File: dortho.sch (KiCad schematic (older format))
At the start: 15 parts, among them SW1 SW_Push, U1 ATmega32U4-AU, Y1 16MHz

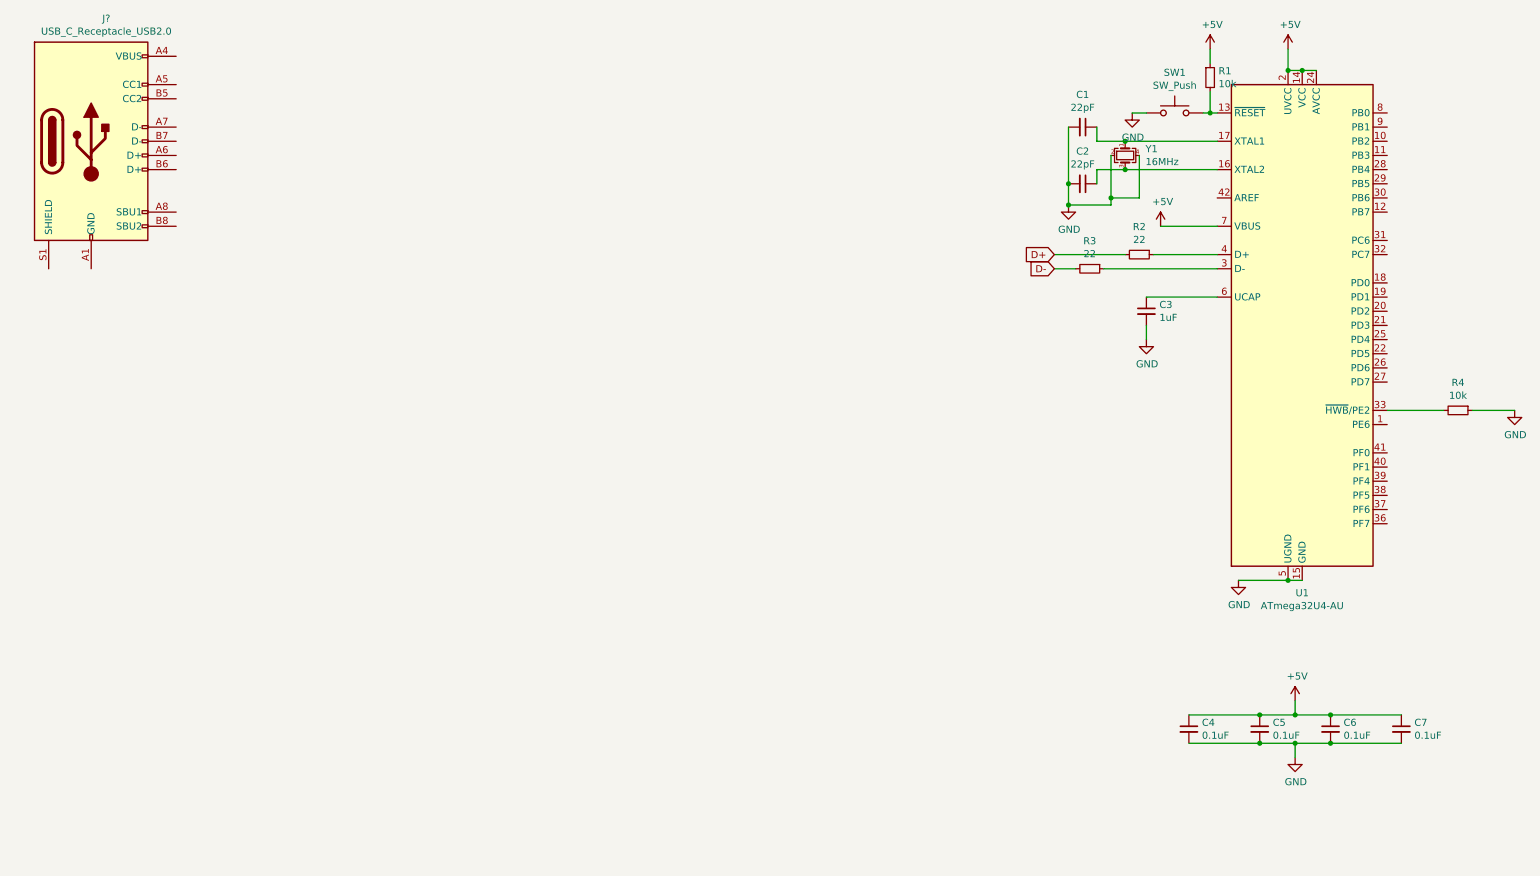
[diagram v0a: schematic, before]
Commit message: Finish switch matrix
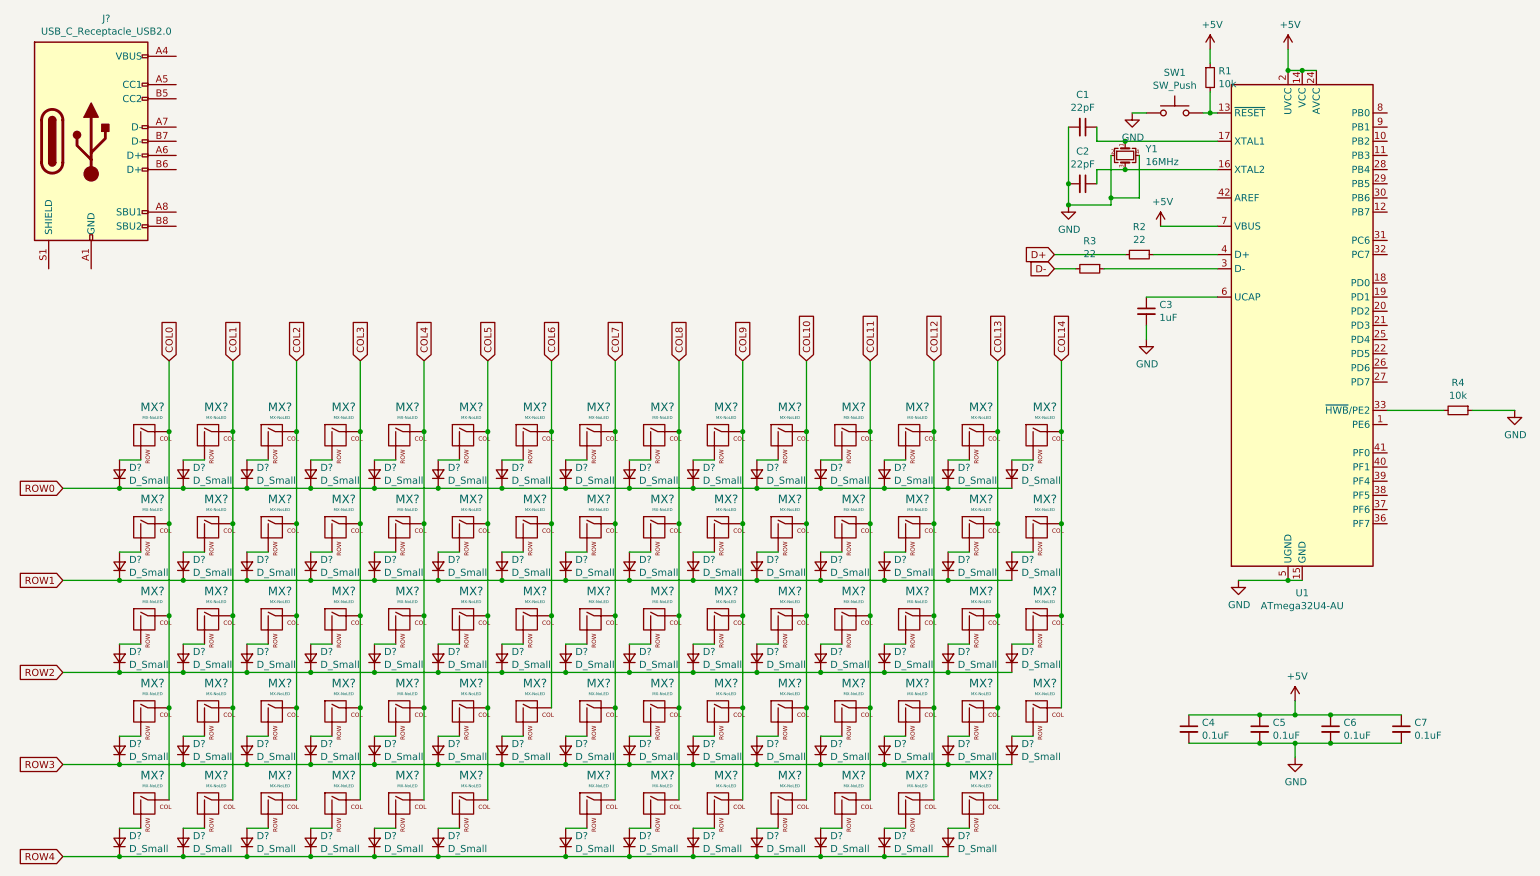
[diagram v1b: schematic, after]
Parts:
- added D? (x73): D_Small, symbol Device:D_Small
- added MX? (x73): MX-NoLED, symbol MX_Alps_Hybrid:MX-NoLED
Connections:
- new net: D?.2 (A), MX?.2 (ROW) (x73)
- new net COL0: MX?.1 (COL), MX?.1 (COL), MX?.1 (COL), MX?.1 (COL), MX?.1 (COL)
- new net COL1: MX?.1 (COL), MX?.1 (COL), MX?.1 (COL), MX?.1 (COL), MX?.1 (COL)
- new net COL10: MX?.1 (COL), MX?.1 (COL), MX?.1 (COL), MX?.1 (COL), MX?.1 (COL)
- new net COL11: MX?.1 (COL), MX?.1 (COL), MX?.1 (COL), MX?.1 (COL), MX?.1 (COL)
- new net COL12: MX?.1 (COL), MX?.1 (COL), MX?.1 (COL), MX?.1 (COL), MX?.1 (COL)
- new net COL13: MX?.1 (COL), MX?.1 (COL), MX?.1 (COL), MX?.1 (COL), MX?.1 (COL)
- new net COL14: MX?.1 (COL), MX?.1 (COL), MX?.1 (COL), MX?.1 (COL)
- new net COL2: MX?.1 (COL), MX?.1 (COL), MX?.1 (COL), MX?.1 (COL), MX?.1 (COL)
- new net COL3: MX?.1 (COL), MX?.1 (COL), MX?.1 (COL), MX?.1 (COL), MX?.1 (COL)
- new net COL4: MX?.1 (COL), MX?.1 (COL), MX?.1 (COL), MX?.1 (COL), MX?.1 (COL)
- new net COL5: MX?.1 (COL), MX?.1 (COL), MX?.1 (COL), MX?.1 (COL), MX?.1 (COL)
- new net COL6: MX?.1 (COL), MX?.1 (COL), MX?.1 (COL), MX?.1 (COL)
- new net COL7: MX?.1 (COL), MX?.1 (COL), MX?.1 (COL), MX?.1 (COL), MX?.1 (COL)
- new net COL8: MX?.1 (COL), MX?.1 (COL), MX?.1 (COL), MX?.1 (COL), MX?.1 (COL)
- new net COL9: MX?.1 (COL), MX?.1 (COL), MX?.1 (COL), MX?.1 (COL), MX?.1 (COL)
- new net ROW0: D?.1 (K), D?.1 (K), D?.1 (K), D?.1 (K), D?.1 (K), D?.1 (K), D?.1 (K), D?.1 (K), D?.1 (K), D?.1 (K), D?.1 (K), D?.1 (K), D?.1 (K), D?.1 (K), D?.1 (K)
- new net ROW1: D?.1 (K), D?.1 (K), D?.1 (K), D?.1 (K), D?.1 (K), D?.1 (K), D?.1 (K), D?.1 (K), D?.1 (K), D?.1 (K), D?.1 (K), D?.1 (K), D?.1 (K), D?.1 (K), D?.1 (K)
- new net ROW2: D?.1 (K), D?.1 (K), D?.1 (K), D?.1 (K), D?.1 (K), D?.1 (K), D?.1 (K), D?.1 (K), D?.1 (K), D?.1 (K), D?.1 (K), D?.1 (K), D?.1 (K), D?.1 (K), D?.1 (K)
- new net ROW3: D?.1 (K), D?.1 (K), D?.1 (K), D?.1 (K), D?.1 (K), D?.1 (K), D?.1 (K), D?.1 (K), D?.1 (K), D?.1 (K), D?.1 (K), D?.1 (K), D?.1 (K), D?.1 (K), D?.1 (K)
- new net ROW4: D?.1 (K), D?.1 (K), D?.1 (K), D?.1 (K), D?.1 (K), D?.1 (K), D?.1 (K), D?.1 (K), D?.1 (K), D?.1 (K), D?.1 (K), D?.1 (K), D?.1 (K)
